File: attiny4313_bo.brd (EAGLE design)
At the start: 49.5 x 22.2 mm, 11 parts, among them J1 AVR_SPI_PRG_6NS, Y1 16MHz

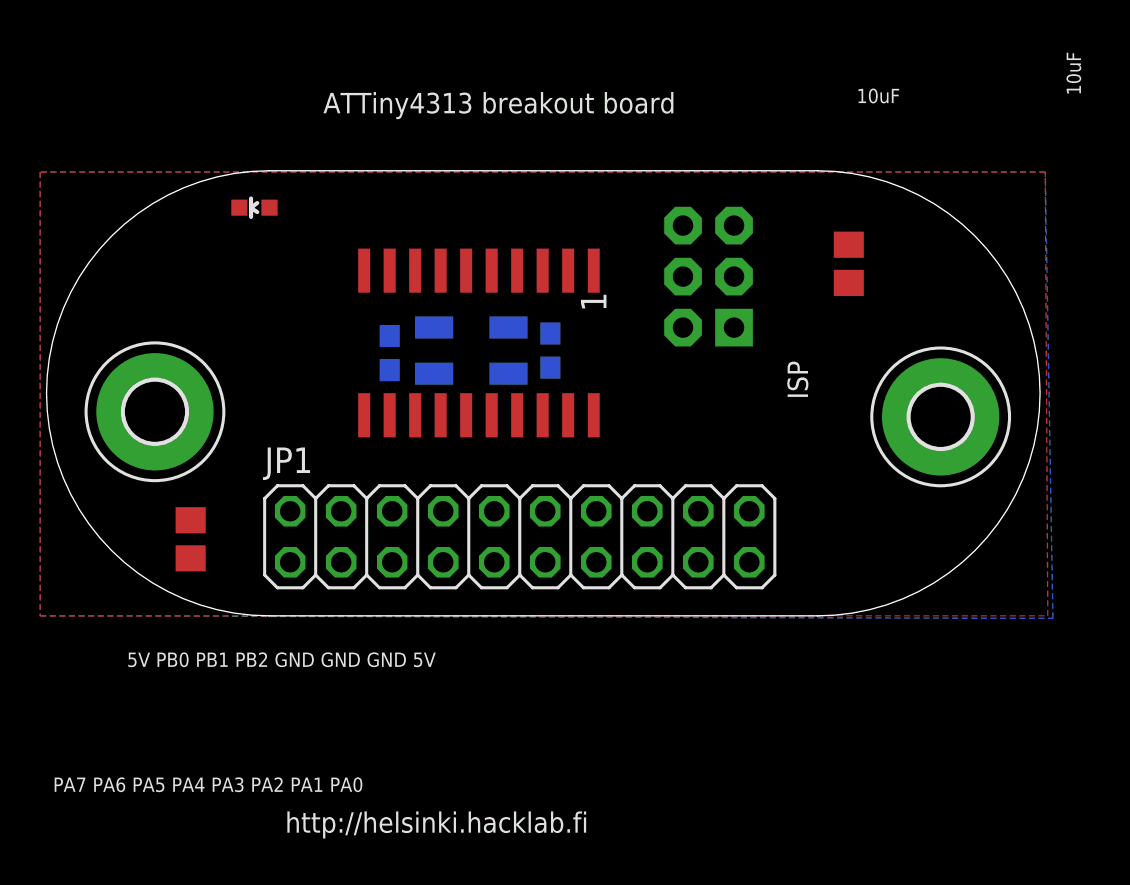
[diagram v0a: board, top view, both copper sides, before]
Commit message: signals v1, probably bad
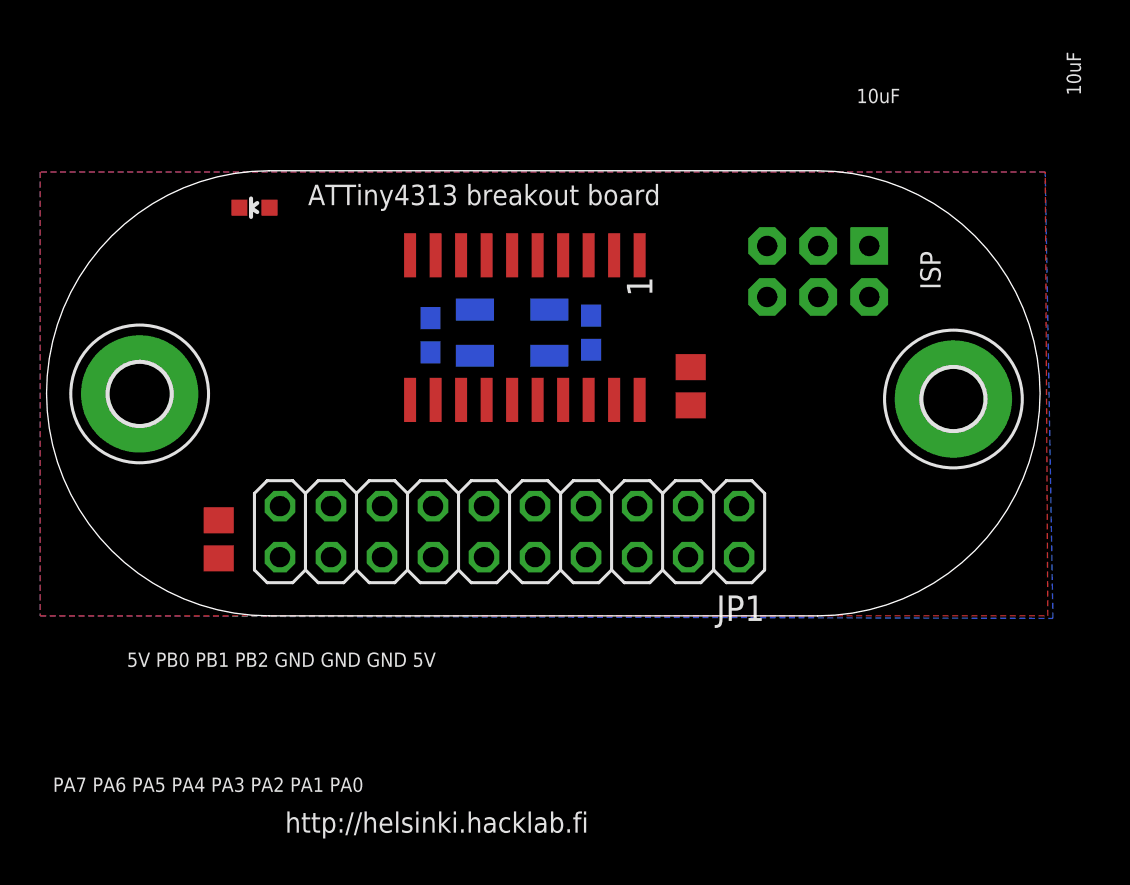
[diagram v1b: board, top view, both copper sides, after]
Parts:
- moved C1 9.96 mm to (32.4, 11.4), turned to 90 degrees
- moved J1 5.47 mm to (38.7, 17.1), turned to 180 degrees
- moved U$1 2.41 mm to (24.1, 14.4)
- moved CX0 2.22 mm to (19.4, 14.0)
- moved CX1 2.22 mm to (27.4, 14.1)
- moved Y1 2.22 mm to (23.5, 14.1)
- moved C2 1.40 mm to (8.89, 3.81), turned to 90 degrees
- moved H1 1.17 mm to (4.95, 11.0)
- moved H2 1.09 mm to (45.5, 10.8)
- moved JP1 0.57 mm to (23.4, 4.19), turned to 180 degrees
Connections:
- removed net N$1: CX0.2, U$1.5, Y1.3
- removed net N$2: LED1.C
- removed net PB0/XTAL1: CX1.2, U$1.4, Y1.1
- new net PA0/XTAL1: CX0.2, JP1.19, U$1.5, Y1.3
- new net PA1/XTAL2: CX1.2, JP1.17, U$1.4, Y1.1
- new net PD0/RDX: JP1.16, U$1.2
- new net PD1/TXD: JP1.14, U$1.3
- new net PD2: JP1.12, U$1.6
- new net PD3: JP1.10, U$1.7
- new net PD4: JP1.8, U$1.8
- new net PD5: JP1.6, U$1.9
- new net PD6: JP1.4, LED1.C, U$1.11
- net +5V: now also JP1.18
- net PB0: now also JP1.15; no longer JP1.1
- net PB1: now also JP1.13; no longer JP1.3
- net PB2: now also JP1.11; no longer JP1.5
- net PB3: now also JP1.9; no longer JP1.7
- net PB4: now also JP1.7; no longer JP1.9
- net PB5/MOSI: now also JP1.5; no longer JP1.13
- net PB6/MISO: now also JP1.3; no longer JP1.11
- net PB7/SCL: now also JP1.1; no longer JP1.15
